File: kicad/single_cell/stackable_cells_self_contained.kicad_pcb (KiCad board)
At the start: 2 copper layers, 20 x 81 mm, 20 parts, among them J1 cell_+, J2 cell_-, J3 bal_even_left, J4 bal_even_right, J5 bal_odd_left, J6 bal_odd_right, Q1 Q_NMOS_DGS, Q2 Q_NMOS_DGS, Q3 Q_NMOS_DGS, U1 FS312F-G, U2 HY2213-xB3y

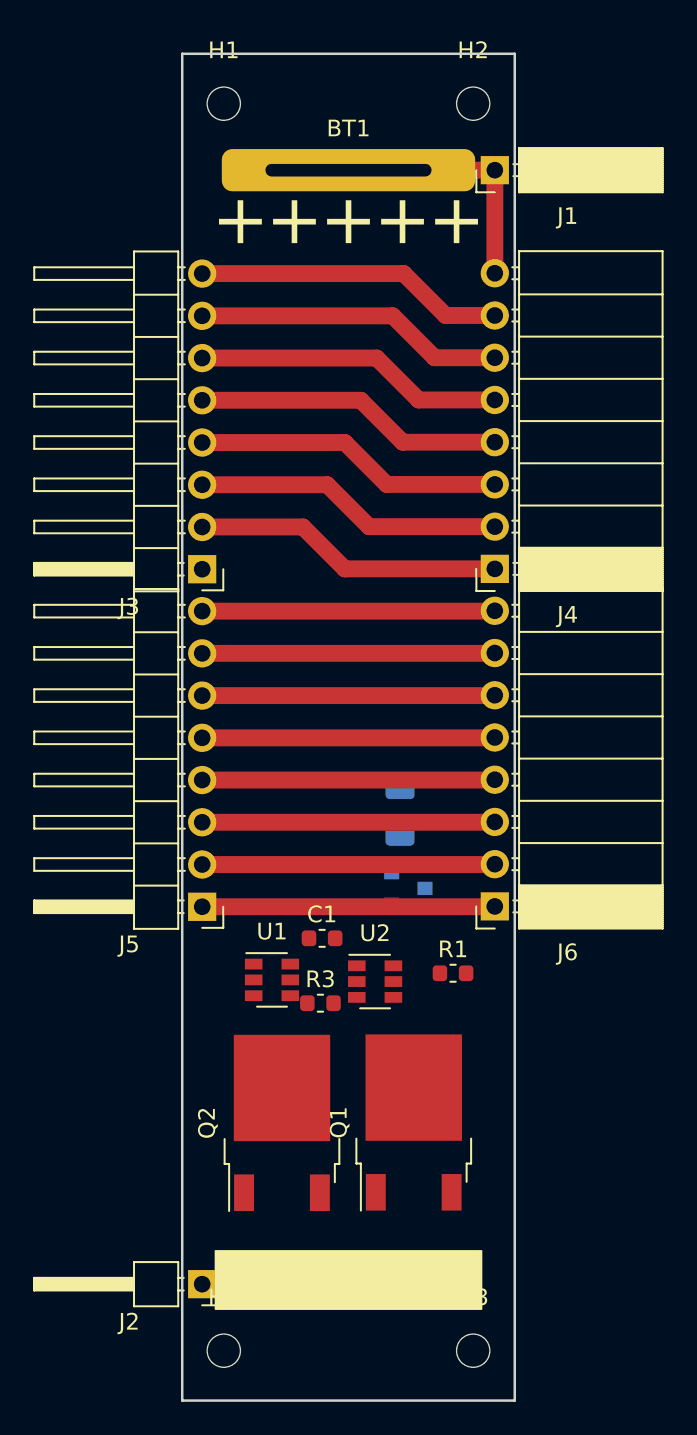
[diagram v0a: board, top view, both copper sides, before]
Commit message: finished stackable design
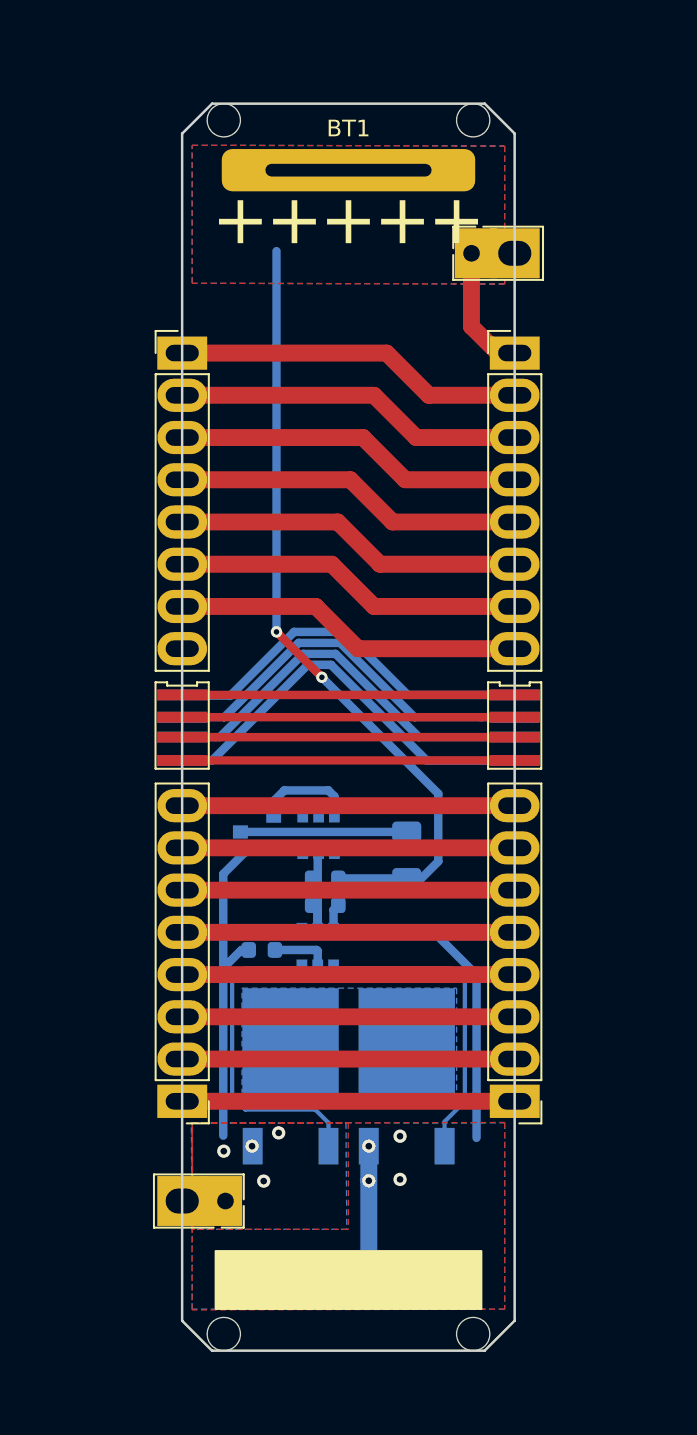
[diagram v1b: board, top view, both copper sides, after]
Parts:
- added J16: communication, telec:DualSide_2x05_P1.27mm_Vertical_SMD, F.Cu at (12.0, 52.6)
- added J17: communication, telec:DualSide_2x05_P1.27mm_Vertical_SMD, F.Cu at (32.0, 52.6)
- C1, R1, R3, U1, U2: moved to B.Cu
- J1: footprint Connector_PinSocket_2.54mm:PinSocket_1x01_P2.54mm_Horizontal -> telec:Castellated_1x01_P5.08mm_Double
- J2: footprint Connector_PinHeader_2.54mm:PinHeader_1x01_P2.54mm_Horizontal -> telec:Castellated_1x01_P5.08mm_Double
- J3, J5: footprint Connector_PinHeader_2.54mm:PinHeader_1x08_P2.54mm_Horizontal -> telec:Castellated_1x08_P2.54mm
- J4, J6: footprint Connector_PinSocket_2.54mm:PinSocket_1x08_P2.54mm_Horizontal -> telec:Castellated_1x08_P2.54mm
- Q1, Q2: value Q_NMOS_DGS -> Q_NMOS_GDS; moved to B.Cu
- Q3: value Q_NMOS_DGS -> Q_NMOS_GSD
- moved J3 13.1 mm to (12.0, 30.0), turned to 0 degrees
- moved J4 13.0 mm to (32.0, 30.0), turned to 0 degrees
- moved J6 11.8 mm to (32.0, 75.0)
- moved J5 11.8 mm to (12.0, 75.0)
- moved Q3 9.71 mm to (16.5, 58.8), turned to 180 degrees
- moved U2 9.62 mm to (20.2, 58.8), turned to 90 degrees
- moved R1 9.57 mm to (20.6, 61.6)
- moved J1 5.14 mm to (32.0, 24.0), turned to 0 degrees
- moved J2 5.14 mm to (12.0, 81.0)
- moved R3 4.76 mm to (16.8, 65.9)
- moved U1 3.29 mm to (20.1, 65.9), turned to 90 degrees
- moved Q2 2.85 mm to (18.5, 73.5)
- moved Q1 2.81 mm to (25.5, 73.5)
- moved R2 2.63 mm to (25.5, 60.2), turned to 90 degrees
- moved C1 2.01 mm to (20.6, 63.2)
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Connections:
- J4 pad 1: Net-(J3-Pad2) -> Net-(BT1-Pad1)
- J4 pad 2: Net-(J3-Pad3) -> Net-(J3-Pad1)
- J4 pad 3: Net-(J3-Pad4) -> Net-(J3-Pad2)
- J4 pad 4: Net-(J3-Pad5) -> Net-(J3-Pad3)
- J4 pad 5: Net-(J3-Pad6) -> Net-(J3-Pad4)
- J4 pad 6: Net-(J3-Pad7) -> Net-(J3-Pad5)
- J4 pad 7: Net-(J3-Pad8) -> Net-(J3-Pad6)
- J4 pad 8: Net-(BT1-Pad1) -> Net-(J3-Pad7)
- Q2 pad 1: Net-(Q1-Pad1) -> Net-(Q2-Pad1)
- Q2 pad 2: Net-(Q2-Pad2) -> Net-(Q1-Pad2)
- Q3 pad 2: Net-(Q3-Pad2) -> Net-(J2-Pad1)
- Q3 pad 3: Net-(J2-Pad1) -> Net-(Q3-Pad3)
- R2 pad 2: Net-(Q3-Pad1) -> Net-(Q3-Pad3)
- U1 pad 1: Net-(Q1-Pad2) -> Net-(Q1-Pad1)
- U1 pad 3: Net-(Q2-Pad2) -> Net-(Q2-Pad1)
- U2 pad 6: Net-(Q3-Pad2) -> Net-(Q3-Pad1)
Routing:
- net Net-(BT1-Pad1): track 15.0 -> 57.5 mm, vias 0 -> 2
- net Net-(J2-Pad1): track 0.00 -> 25.8 mm, vias 0 -> 4
- net Net-(J16-Pad8): track 0.00 -> 24.3 mm
- net Net-(J16-Pad6): track 0.00 -> 23.7 mm
- net Net-(J16-Pad4): track 0.00 -> 23.2 mm
- net Net-(J16-Pad2): track 0.00 -> 22.7 mm
- net Net-(BT1-Pad2): track 8.80 -> 30.0 mm, vias 0 -> 4
- net Net-(J3-Pad1): track 0.00 -> 21.1 mm
- net Net-(J16-Pad7): track 0.00 -> 20.0 mm
- net Net-(J16-Pad5): track 0.00 -> 20.0 mm
- net Net-(J16-Pad3): track 0.00 -> 20.0 mm
- net Net-(J16-Pad1): track 0.00 -> 20.0 mm
- net Net-(Q2-Pad1): track 0.00 -> 19.3 mm
- net Net-(J3-Pad8): track 18.6 -> 0.00 mm
- net Net-(Q1-Pad1): track 0.00 -> 18.6 mm
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- added copper zone on B.Cu, net Net-(BT1-Pad1)
- added copper zone on F.Cu, net Net-(BT1-Pad1)
- added copper zone on B.Cu, net Net-(BT1-Pad2)
- added copper zone on F.Cu, net Net-(BT1-Pad2)
- added copper zone on B.Cu, net Net-(J2-Pad1)
- added copper zone on F.Cu, net Net-(J2-Pad1)
- added copper zone on B.Cu, net Net-(Q1-Pad2)
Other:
- board size 20 x 81 mm -> 20 x 75 mm
- board text added: "telec 2021"

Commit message: Updated to kicad 7.x
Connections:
- J3 pad 8: Net-(J3-Pad8) -> unconnected-(J3-Pin_8-Pad8)
- U1 pad 4: Net-(U1-Pad4) -> unconnected-(U1-TD-Pad4)
- U2 pad 1: Net-(U2-Pad1) -> unconnected-(U2-NC-Pad1)
- U2 pad 4: Net-(U2-Pad4) -> unconnected-(U2-NC-Pad4)
- U2 pad 5: Net-(U2-Pad5) -> unconnected-(U2-NC-Pad5)
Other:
- net class Default removed
